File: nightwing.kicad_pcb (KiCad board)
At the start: 2 copper layers, 165.4 x 129.6 mm, 109 parts, among them J1 USB_C_Receptacle_USB2.0, J2 USB_C_Receptacle_USB2.0, J3 OLED, SW1 SW_PUSH, SW10 SW_PUSH, SW11 SW_PUSH, SW12 SW_PUSH, SW13 SW_PUSH, SW14 SW_PUSH, SW15 SW_PUSH, SW16 SW_PUSH, SW17 SW_PUSH, SW18 SW_PUSH, SW19 Rotary_Encoder, SW2 SW_PUSH, SW20 SW_PUSH, SW21 SW_PUSH, SW22 SW_PUSH, SW23 SW_PUSH, SW24 SW_PUSH, SW3 SW_PUSH, SW4 SW_PUSH, SW5 SW_PUSH, SW6 SW_PUSH, SW7 SW_PUSH, SW8 SW_PUSH, SW9 SW_PUSH, U1 PRTR5V0U2X, U3 ATmega32U4-AU, X1 16mhz

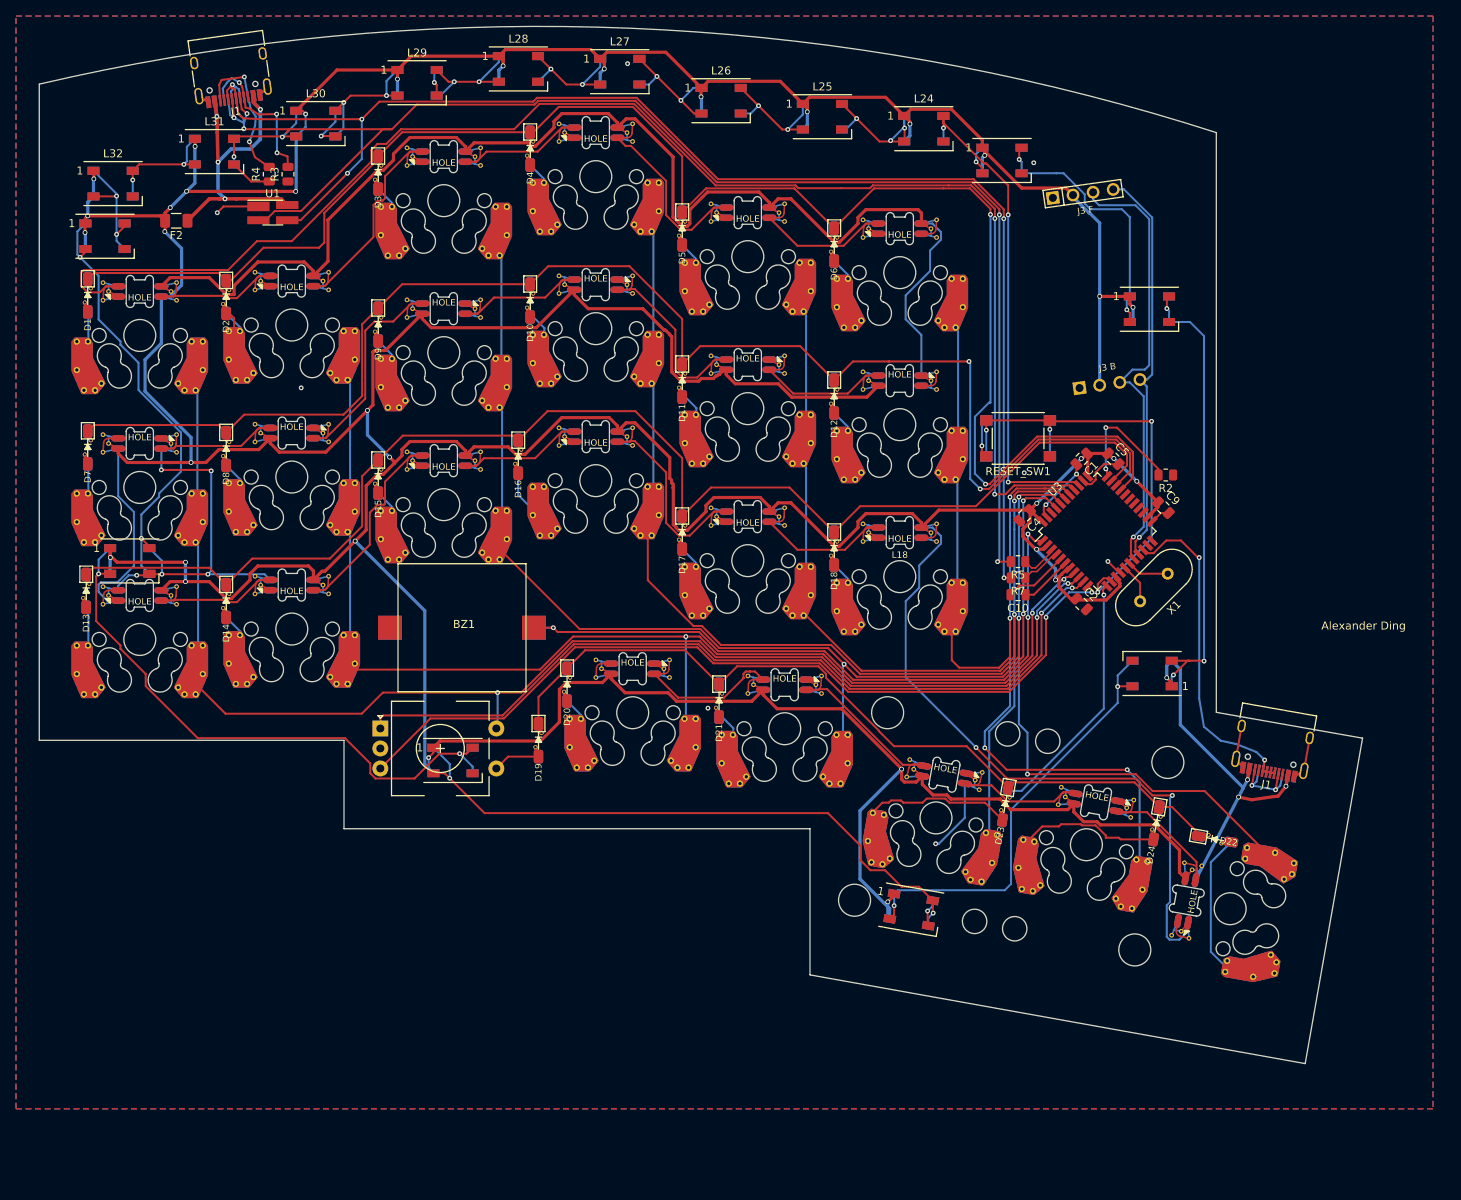
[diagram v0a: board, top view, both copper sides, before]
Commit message: updated stm32
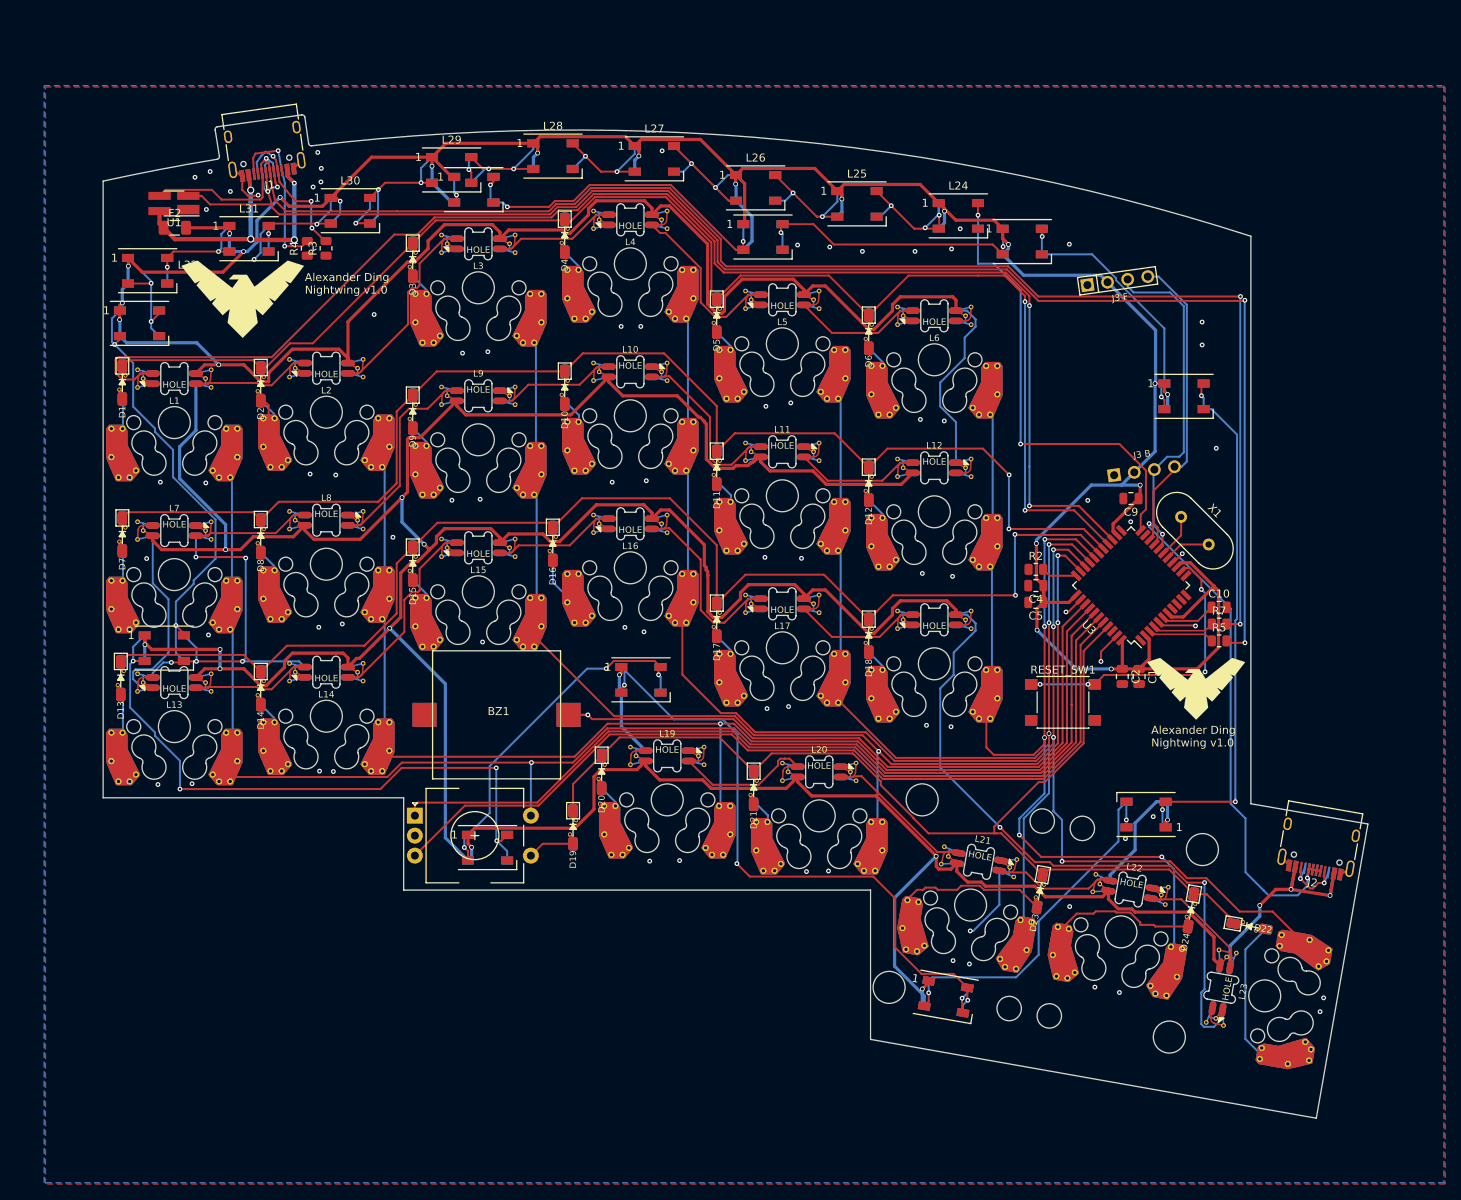
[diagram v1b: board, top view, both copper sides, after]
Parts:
- added G***: LOGO, private:tiny_nightwing, F.Cu at (37.1, 38.7)
- added G***: LOGO, private:icon_nightwing, F.Cu at (156.2, 87.4)
- added L40: WS2812B, reversible-kicad-footprints:ws2812_reversible, B.Cu at (86.9, 86.4)
- added L41: WS2812B, reversible-kicad-footprints:ws2812_reversible, B.Cu at (102.1, 31.0)
- added L42: WS2812B, reversible-kicad-footprints:ws2812_reversible, B.Cu at (66.0, 25.1)
- J2: moved to F.Cu
- moved RESET_SW1 33.5 mm to (139.6, 89.2)
- moved C1 28.1 mm to (149.1, 86.0), turned to 270 degrees
- moved R5 27.0 mm to (159.1, 81.5), turned to 0 degrees
- moved R7 25.8 mm to (159.1, 79.4), turned to 0 degrees
- moved C10 25.2 mm to (159.1, 77.3), turned to 0 degrees
- moved C5 20.4 mm to (136.2, 76.7), turned to 180 degrees
- moved R2 20.1 mm to (136.2, 72.6), turned to 0 degrees
- moved L37 17.6 mm to (150.0, 103.2)
- moved J2 13.5 mm to (171.8, 106.2), turned to 170 degrees
- moved U1 12.4 mm to (28.5, 26.8), turned to 180 degrees
- moved D23 11.7 mm to (136.7, 112.8)
- moved L16 11.7 mm to (85.5, 66.9)
- moved L17 11.7 mm to (104.5, 76.9)
- moved L18 11.7 mm to (123.5, 78.9)
- moved SW12 11.7 mm to (123.5, 65.4)
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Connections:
- L36 pad 4: Net-(L35-Pad2) -> Net-(L36-Pad4)
- U3 pad 1: BUZZER -> (no net)
- U3 pad 10: ROT_A -> (no net)
- U3 pad 11: ROT_B -> (no net)
- U3 pad 12: ROW3 -> (no net)
- U3 pad 21: Net-(U3-Pad21) -> (no net)
- U3 pad 22: Net-(U3-Pad22) -> WS_LED
- U3 pad 25: Net-(U3-Pad25) -> SK_LED
- U3 pad 26: Net-(U3-Pad26) -> ROW0
- U3 pad 27: Net-(U3-Pad27) -> ROW1
- U3 pad 28: Net-(U3-Pad28) -> ROW2
- U3 pad 29: Net-(U3-Pad29) -> COL5
- U3 pad 30: ROW0 -> COL4
- U3 pad 31: ROW1 -> COL3
- U3 pad 32: ROW2 -> COL2
- U3 pad 36: WS_LED -> BUZZER
- U3 pad 37: SK_LED -> COL1
- U3 pad 38: COL5 -> COL0
- U3 pad 39: COL4 -> ROT_A
- U3 pad 40: COL3 -> ROT_B
- U3 pad 41: COL2 -> ROW3
- U3 pad 42: Net-(U3-Pad42) -> (no net)
- U3 pad 8: COL1 -> (no net)
- U3 pad 9: COL0 -> (no net)
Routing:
- net Net-(L36-Pad4): track 0.00 -> 80.0 mm, vias 0 -> 3
- net +5V: track 983.4 -> 1041.2 mm, vias 38 -> 36
- net Net-(L41-Pad2): track 0.00 -> 42.7 mm, vias 0 -> 3
- net Net-(L35-Pad2): track 78.2 -> 43.8 mm, vias 2 -> 3
- net GND: track 143.7 -> 111.2 mm, vias 21 -> 88
- net Net-(L39-Pad2): track 3.85 -> 35.7 mm, vias 1 -> 2
- net ROW0: track 204.0 -> 176.9 mm
- net DP: track 177.1 -> 200.6 mm, vias 5 -> 3
- net RX: track 44.6 -> 66.6 mm
- net ROW1: track 180.1 -> 158.4 mm
- net RESET: track 57.1 -> 39.3 mm
- net DN: track 183.3 -> 199.0 mm, vias 5 -> 4
- net SCL: track 56.6 -> 42.3 mm
- net SDA: track 50.7 -> 38.9 mm, vias 1 -> 0
- net Net-(R2-Pad2): track 15.6 -> 4.47 mm, vias 2 -> 0
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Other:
- board size 165.4 x 129.6 mm -> 158.1 x 125.4 mm
- board text added: "Nightwing v1.0"
